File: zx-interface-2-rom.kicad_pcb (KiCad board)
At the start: 4 copper layers, 39.4 x 50.1 mm, 9 parts, among them J1 cartridge_IF2, SW1 SW_DIP_x02, U1 W27C512, U2 74LS32

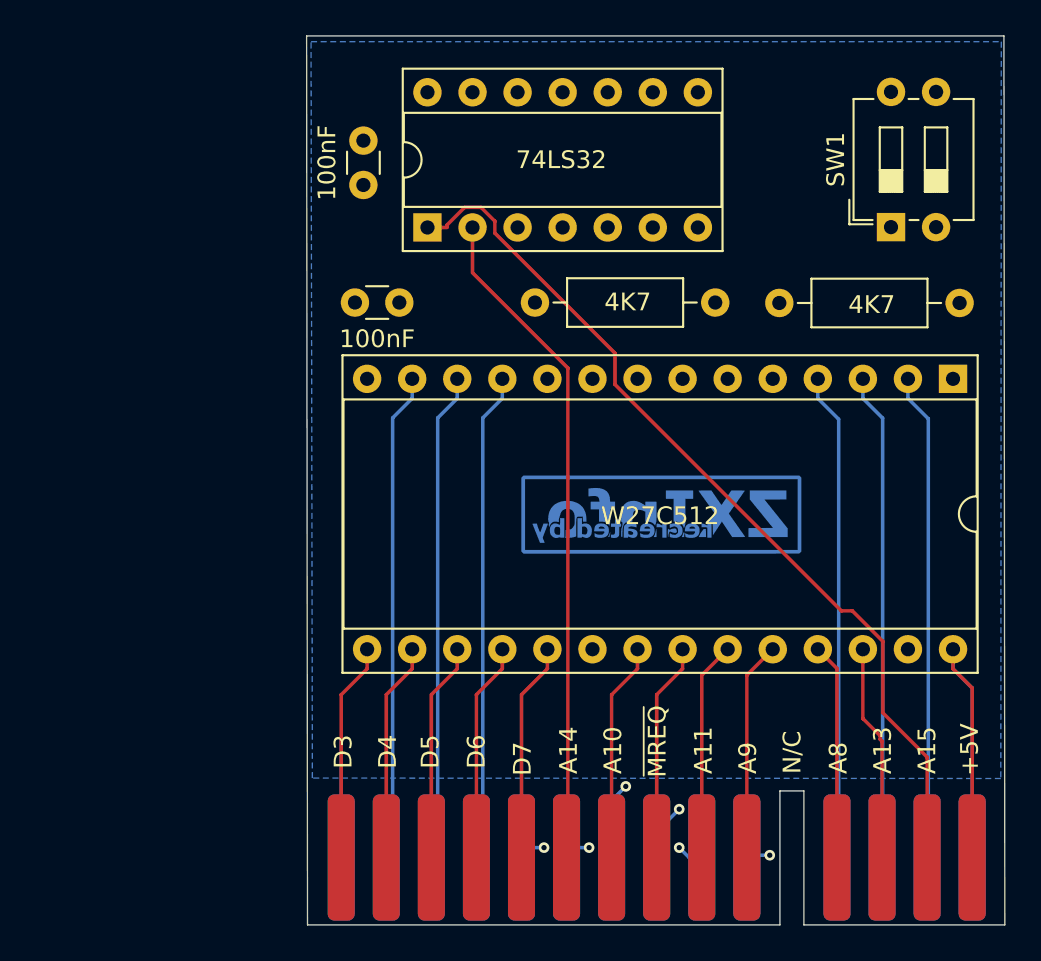
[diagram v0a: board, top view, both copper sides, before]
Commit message: Updated SYMBOL & FOOTPRINT library
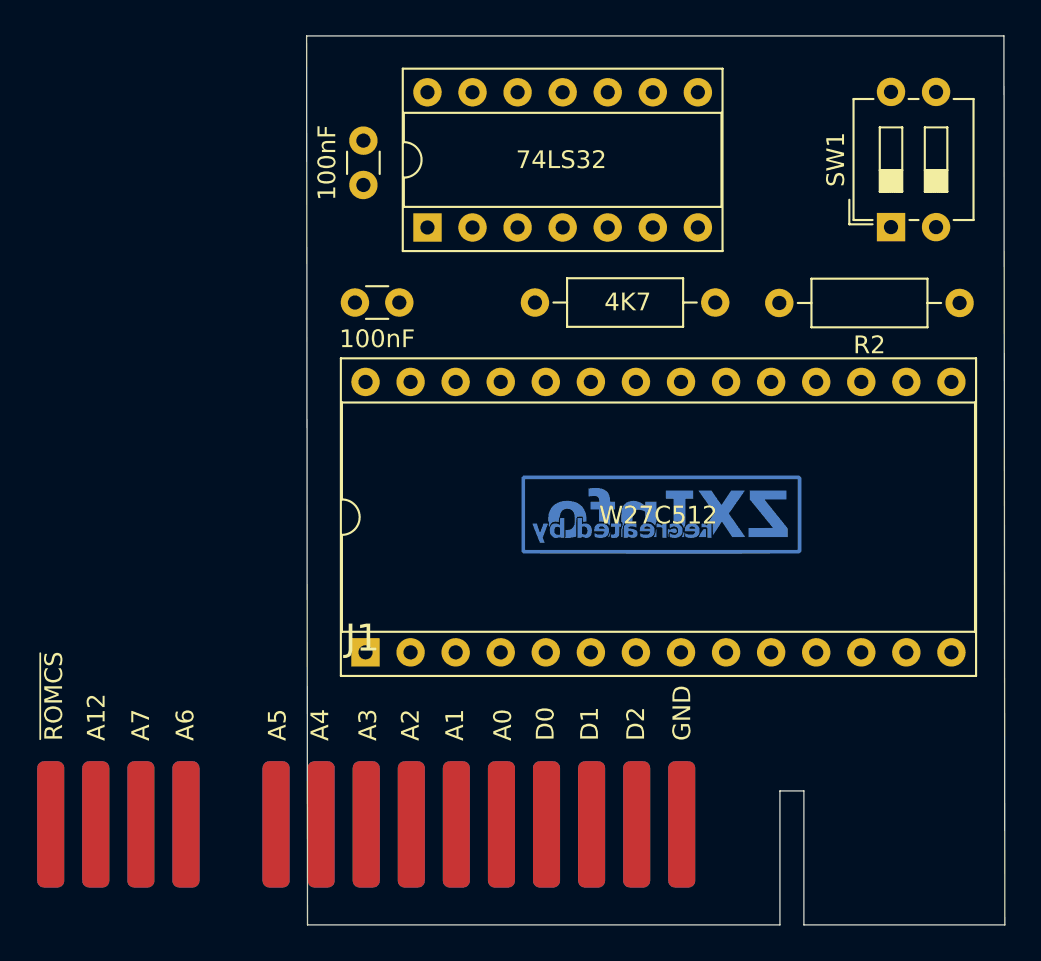
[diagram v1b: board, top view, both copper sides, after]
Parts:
- G200: footprint ZXINFO_LIB:ZXInfo_kicad_logo_copper_16.5x5 -> ZXINFO_FOOTPRINT:ZXInfo_kicad_logo_copper_16.5x5
- J1: footprint ZXINFO_LIB:CART_IF2_EDGE -> ZXINFO_FOOTPRINT:CART_IF2_EDGE; moved to F.Cu
- moved U1 36.5 mm to (87.1, 80.7), turned to 90 degrees
- moved J1 31.7 mm to (79.5, 90.4), turned to 0 degrees
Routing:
- net +5V: track 95.1 -> 0.00 mm
- net Net-(J1-A15): track 51.0 -> 0.00 mm
- net Net-(U1-A15): track 42.9 -> 0.00 mm
- net Net-(J1-~{MREQ}): track 41.8 -> 0.00 mm
- net Net-(J1-A14): track 37.8 -> 0.00 mm
- net Net-(U1-A14): track 37.0 -> 0.00 mm
- net A4: track 29.1 -> 0.00 mm, vias 1 -> 0
- net A5: track 29.0 -> 0.00 mm, vias 1 -> 0
- net A0: track 28.8 -> 0.00 mm, vias 1 -> 0
- net A1: track 28.8 -> 0.00 mm, vias 1 -> 0
- net A3: track 28.3 -> 0.00 mm, vias 1 -> 0
- net A2: track 28.0 -> 0.00 mm, vias 1 -> 0
- net D1: track 27.6 -> 0.00 mm
- net D2: track 27.6 -> 0.00 mm
- net D0: track 27.6 -> 0.00 mm
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- removed copper zone on B.Cu, net GND
